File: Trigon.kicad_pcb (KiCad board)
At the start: 2 copper layers, 160 x 120 mm, 72 parts, among them J1 USB_C_Receptacle_USB2.0, SW1 SW_Push, SW2 Rotary_Encoder_Switch, U1 ATmega32U4-AU, Y1 16MHz

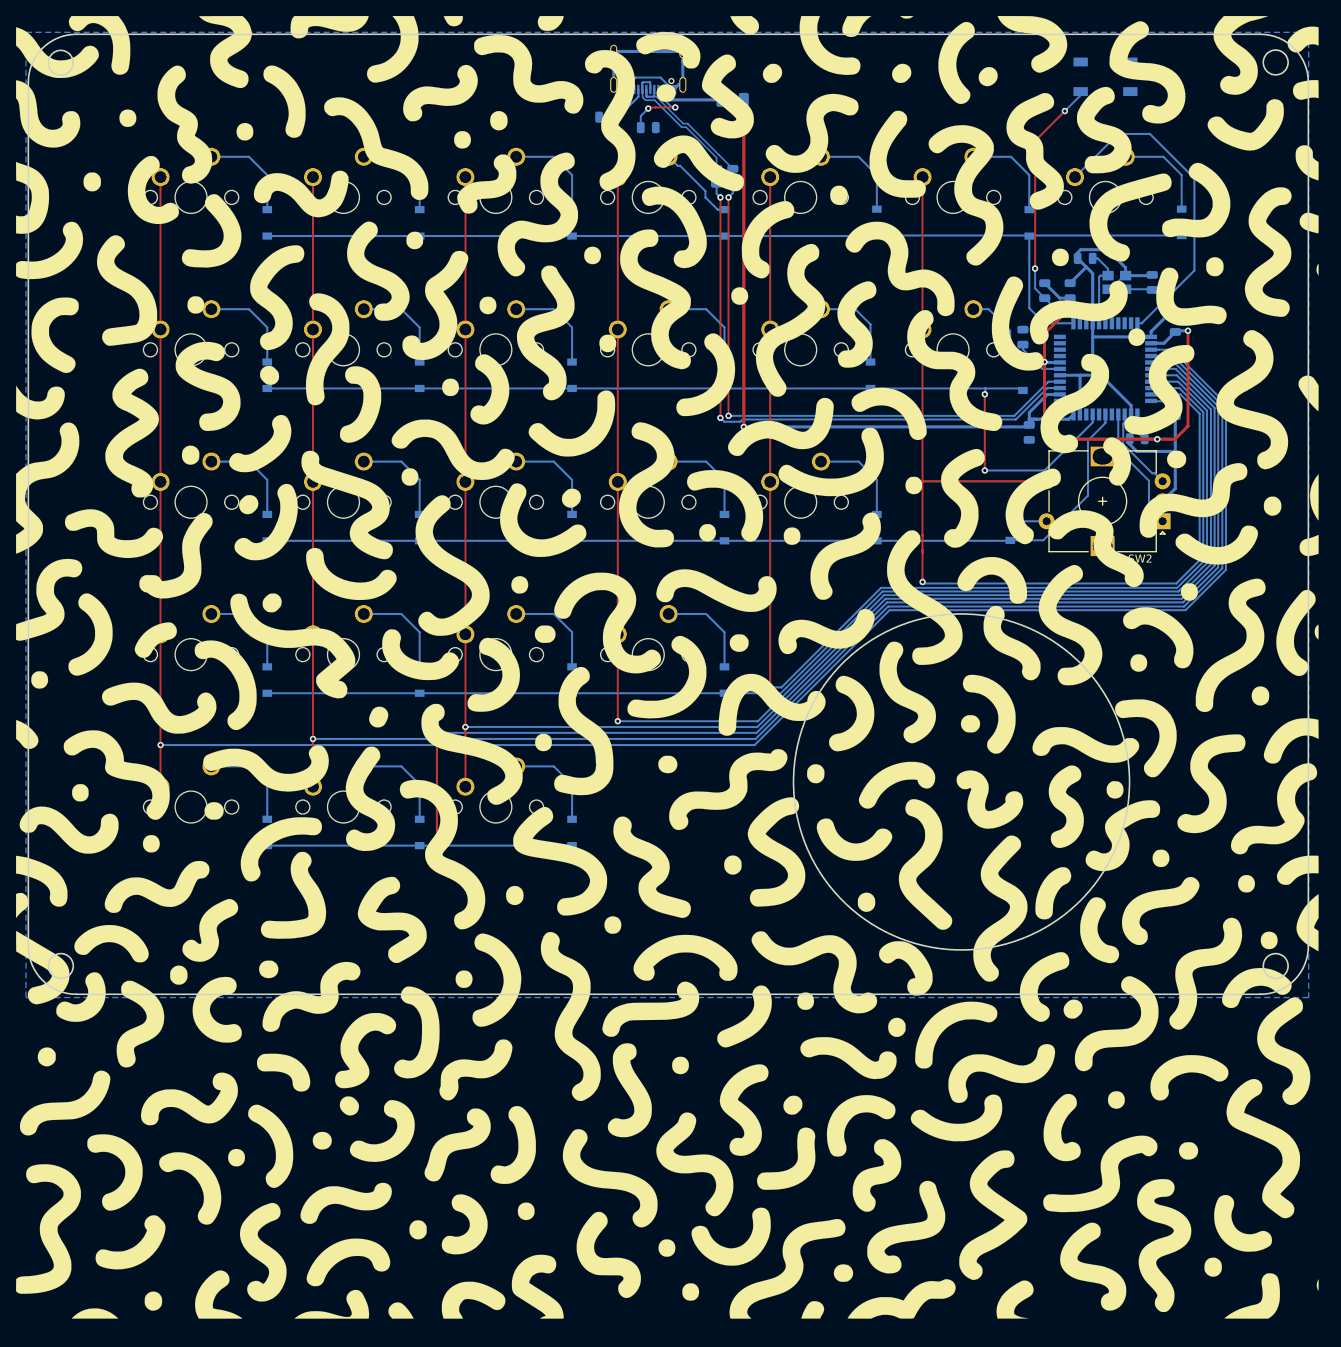
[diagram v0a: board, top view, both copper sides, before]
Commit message: new usb connector'
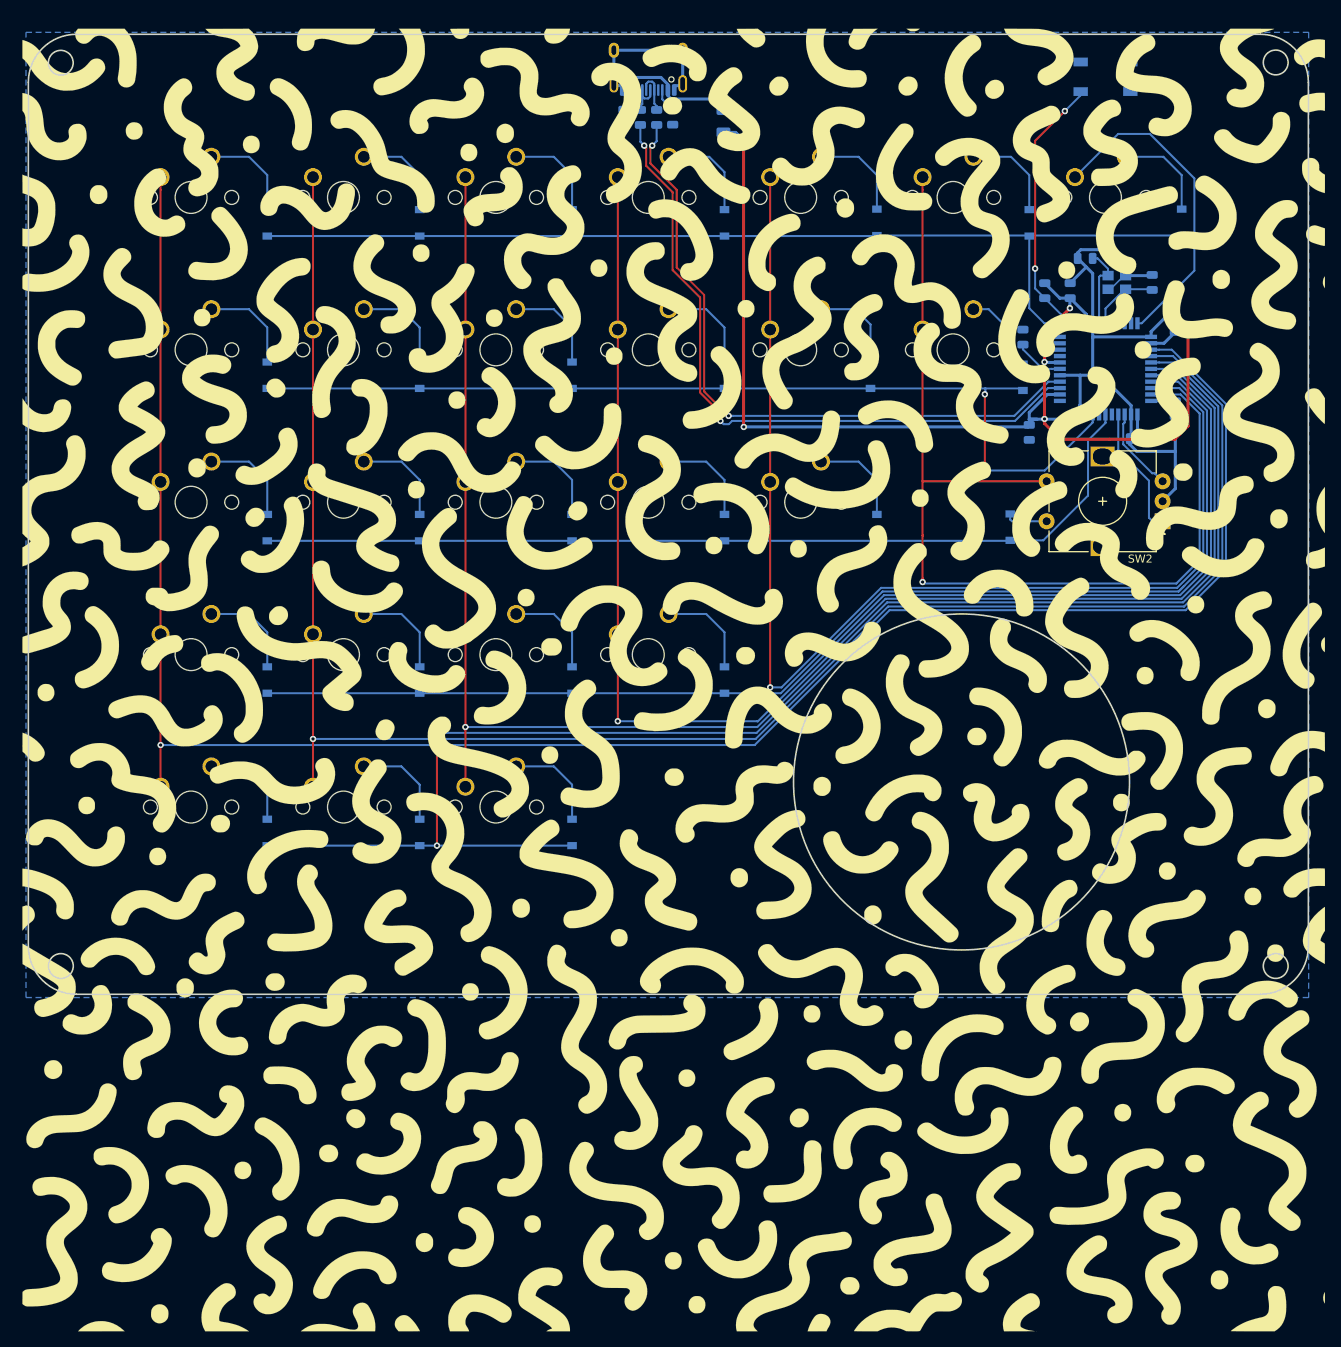
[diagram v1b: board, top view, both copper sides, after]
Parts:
- F1: value Polyfuse_Small -> 500mA
- J1: value USB_C_Receptacle_USB2.0 -> TYPE-C-31-M12_13; footprint Connector_USB:USB_C_Receptacle_Palconn_UTC16-G -> acheron_Connectors:TYPE-C-31-M-12
- moved G*** 19.8 mm to (78.6, -55.6)
- moved R1 12.0 mm to (77.2, -105.3)
- moved R2 12.0 mm to (75.2, -105.3)
- moved R5 3.31 mm to (79.2, -105.3), turned to 90 degrees
- moved J1 3.30 mm to (76.2, -108.0)
- moved F1 2.90 mm to (85.6, -104.8), turned to 90 degrees
- moved R4 2.16 mm to (73.2, -105.3), turned to 90 degrees
- moved G*** 1.77 mm to (79.4, -34.9)
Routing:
- net D+: track 18.1 -> 4.94 mm
- net Net-(R2-Pad1): track 73.8 -> 85.6 mm
- net Net-(R1-Pad1): track 72.4 -> 83.9 mm
- net D-: track 17.5 -> 7.03 mm
- net Net-(J1-PadB5): track 9.38 -> 3.54 mm, vias 2 -> 0
- net Net-(D4-Pad2): track 10.2 -> 12.5 mm
- net +5V: track 158.3 -> 156.2 mm
- net Net-(J1-PadA5): track 5.01 -> 3.83 mm
- net VCC: track 14.6 -> 15.2 mm

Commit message: latest
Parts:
- moved G*** 128.6 mm to (92.6, 72.3), turned to 180 degrees
- moved C1 128.5 mm to (152.7, 43.2)
- moved C4 128.5 mm to (155.6, 48.4)
- moved C5 128.5 mm to (150.8, 62.7)
- moved C6 128.5 mm to (142.4, 44.2)
- moved D1 128.5 mm to (42.1, 35.7)
- moved D10 128.5 mm to (80.2, 54.8)
- moved D11 128.5 mm to (99.2, 54.8)
- moved D12 128.5 mm to (117.5, 54.8)
- moved D13 128.5 mm to (136.5, 55.0)
- moved D19 128.5 mm to (42.1, 92.9)
- moved D2 128.5 mm to (61.1, 35.7)
- moved D20 128.5 mm to (61.1, 92.9)
- moved D21 128.5 mm to (80.2, 92.9)
- moved D22 128.5 mm to (99.2, 92.9)
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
